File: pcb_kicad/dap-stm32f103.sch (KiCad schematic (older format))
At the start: 35 parts, among them J1 USB_C_Receptacle_USB2.0, U1 STM32F103CBTx, Y1 SMD-5032_2P_8MHz_20ppm_20pF

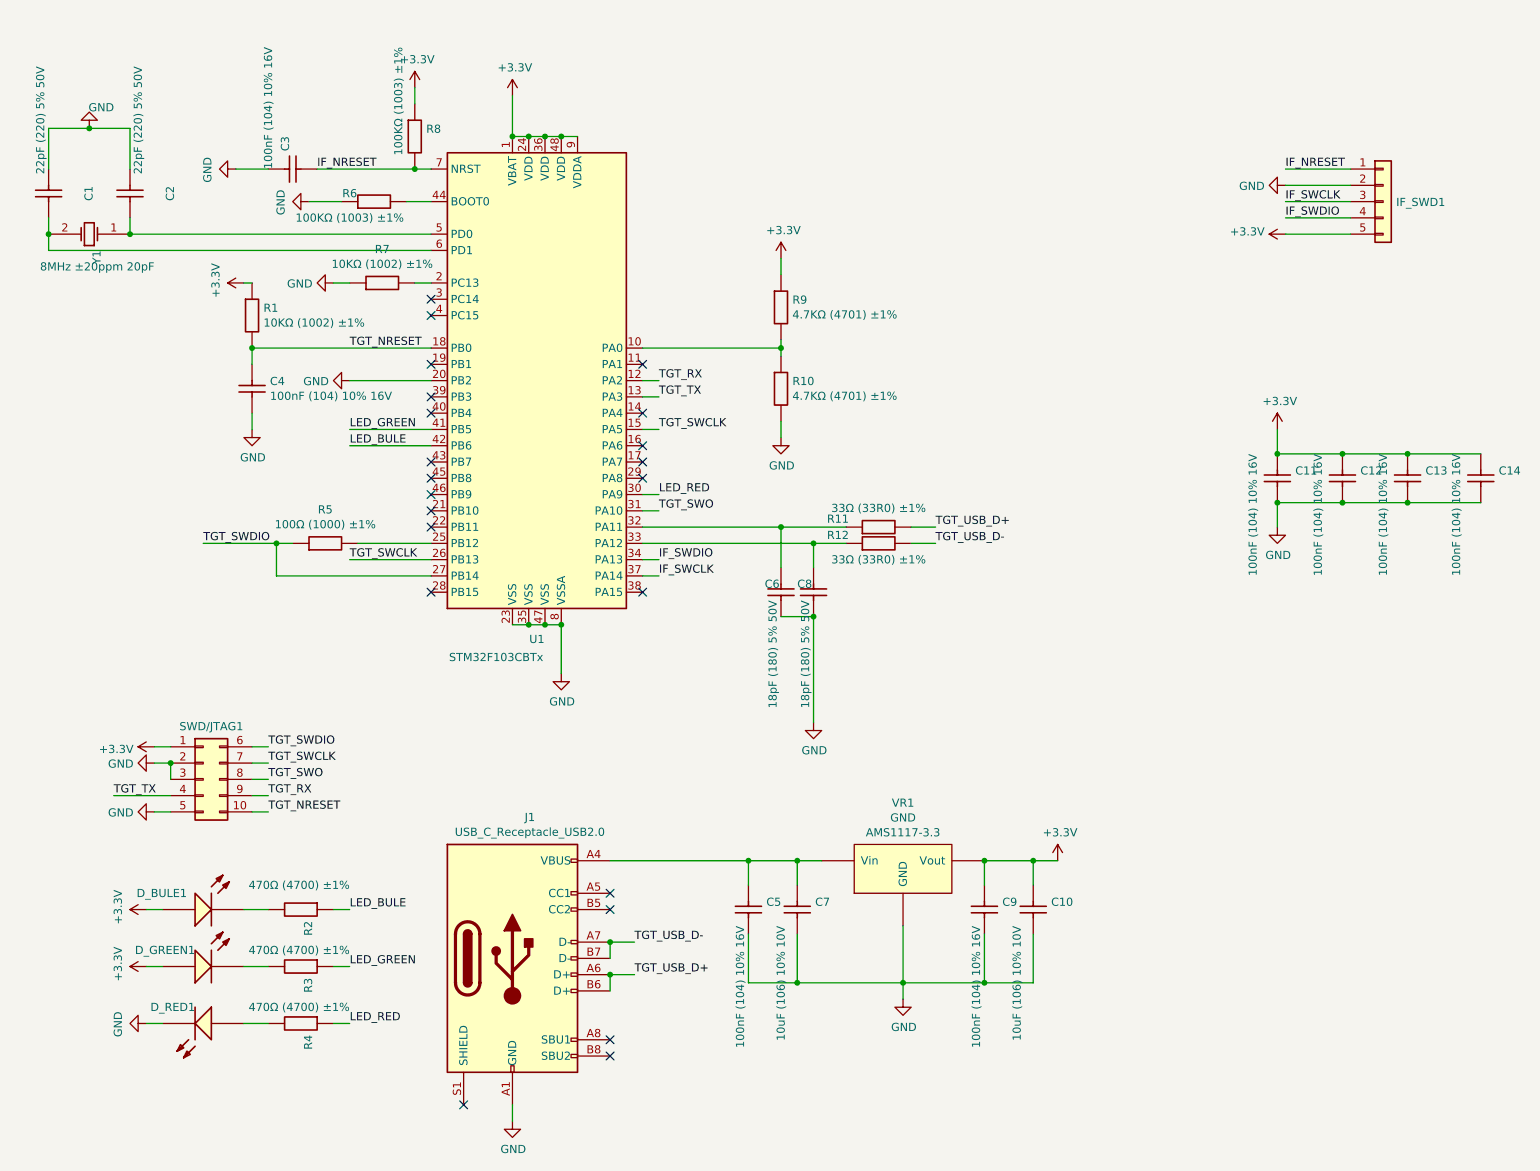
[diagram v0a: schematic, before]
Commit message: [update] pcb
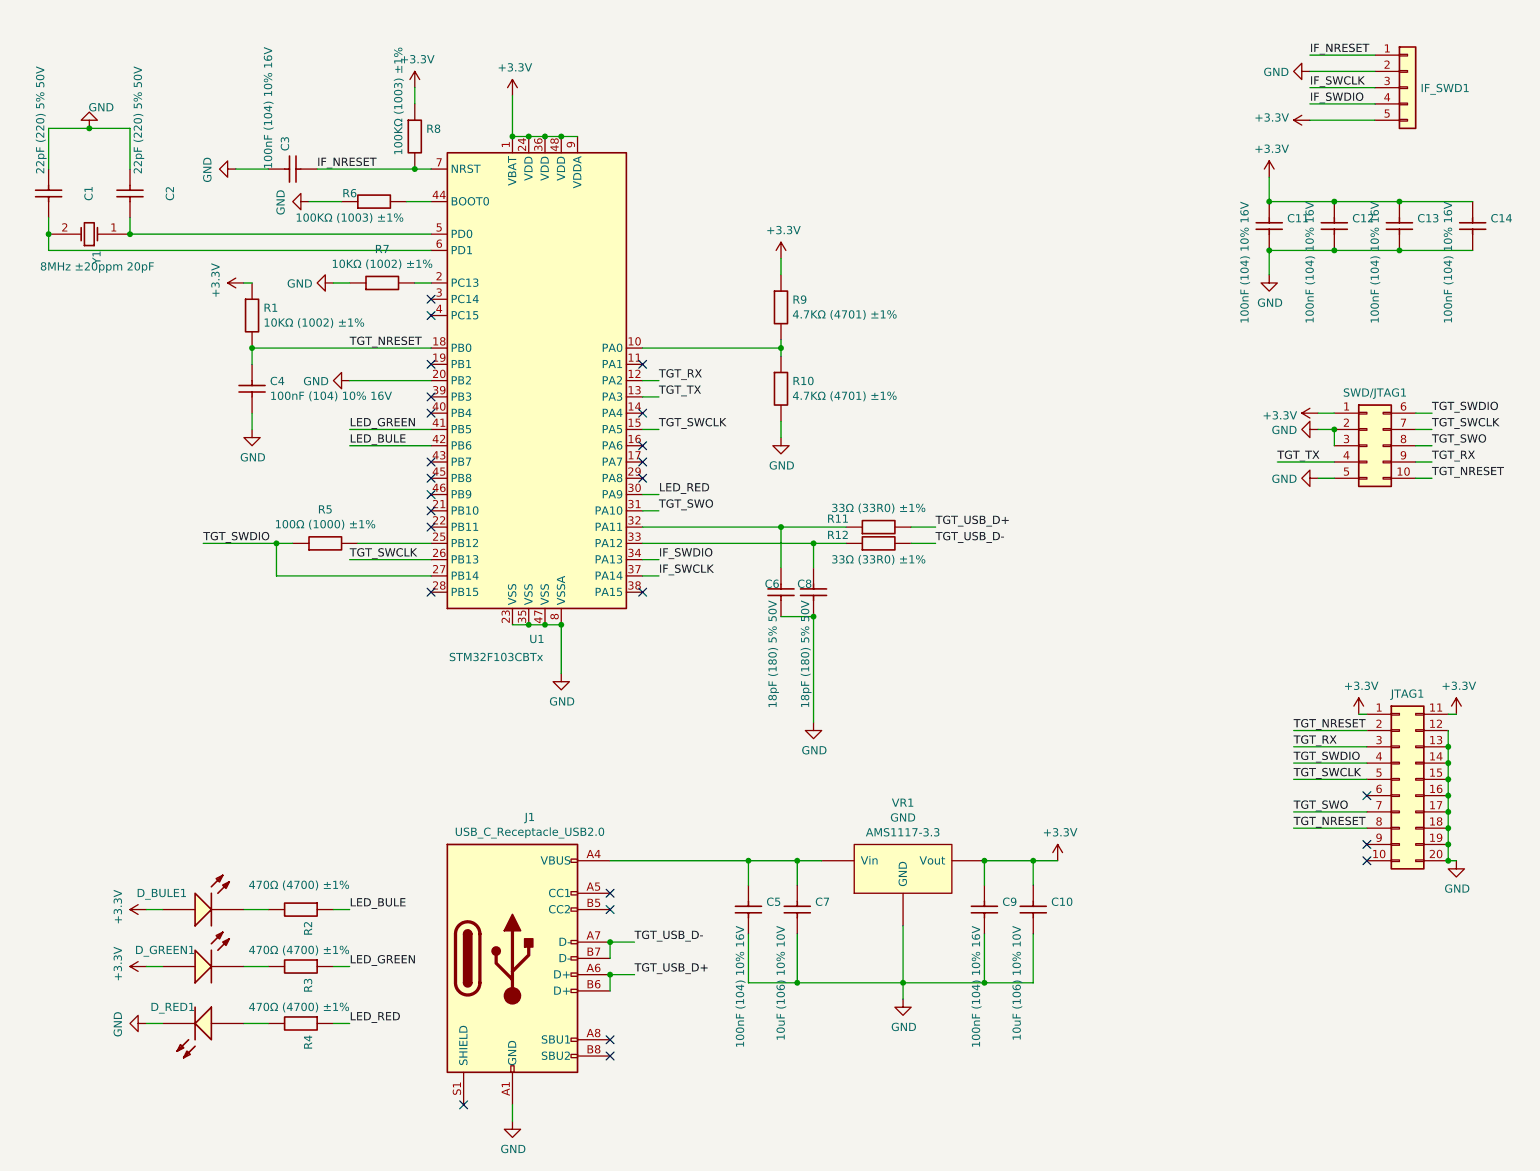
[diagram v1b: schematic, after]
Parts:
- added JTAG1: Conn_02x10_Top_Bottom, Connector_PinHeader_2.54mm:PinHeader_2x10_P2.54mm_Vertical, symbol Connector_Generic:Conn_02x10_Top_Bottom
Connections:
- net +3V3: now also JTAG1.1 (Pin_1), JTAG1.11 (Pin_11)
- net GND: now also JTAG1.12 (Pin_12), JTAG1.13 (Pin_13), JTAG1.14 (Pin_14), JTAG1.15 (Pin_15), JTAG1.16 (Pin_16), JTAG1.17 (Pin_17), JTAG1.18 (Pin_18), JTAG1.19 (Pin_19), JTAG1.20 (Pin_20)
- net TGT_NRESET: now also JTAG1.2 (Pin_2), JTAG1.8 (Pin_8)
- net TGT_RX: now also JTAG1.3 (Pin_3)
- net TGT_SWCLK: now also JTAG1.5 (Pin_5)
- net TGT_SWDIO: now also JTAG1.4 (Pin_4)
- net TGT_SWO: now also JTAG1.7 (Pin_7)
- no-connect marks 22 -> 25
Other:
- moved on the sheet: C11, C12, C13, C14, IF_SWD1, SWD/JTAG1
